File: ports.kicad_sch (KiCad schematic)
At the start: 6 parts, among them J1 PCA9865 2, J12 I2C, J2 I2S, J4 IMU, J6 Expansion

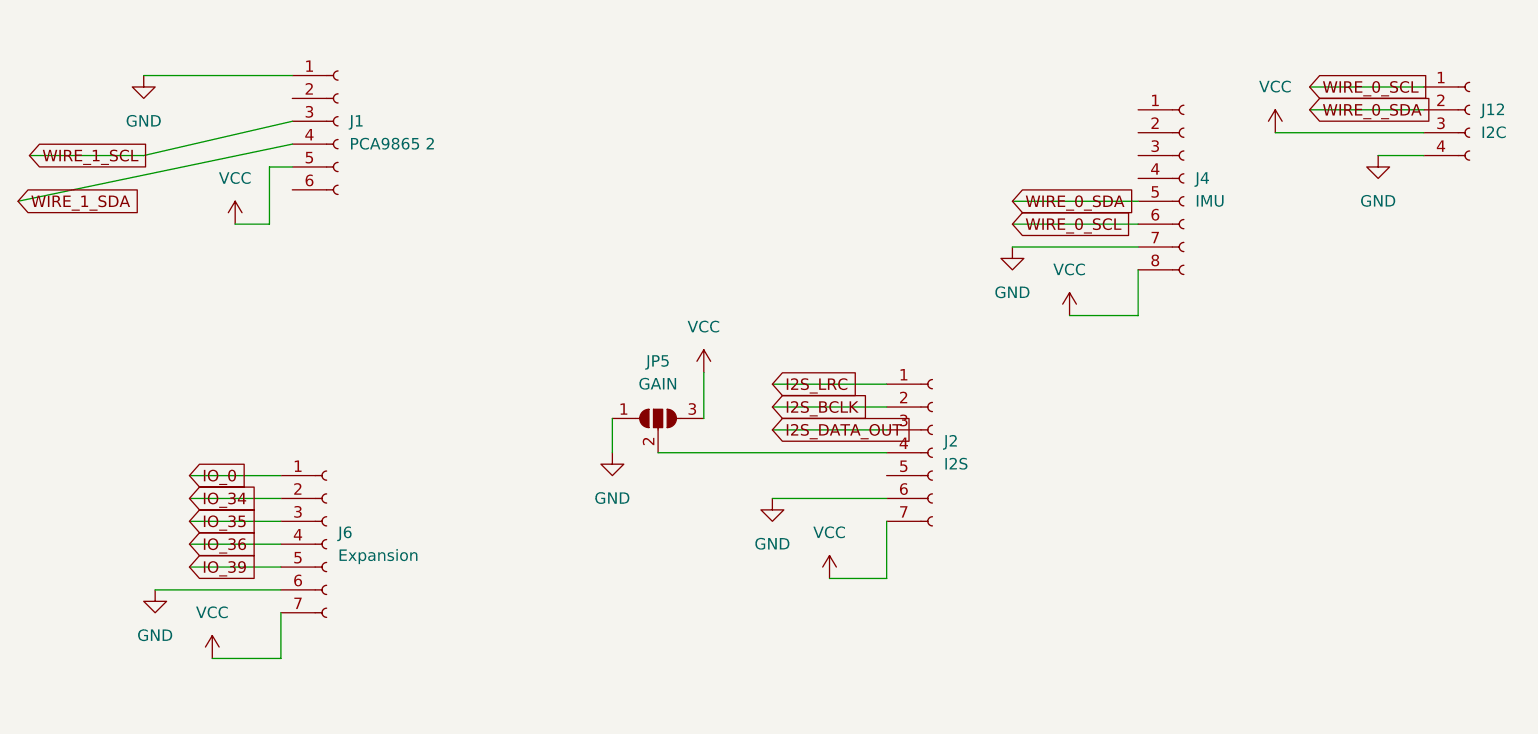
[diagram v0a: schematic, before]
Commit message: Cleaned revision 2.
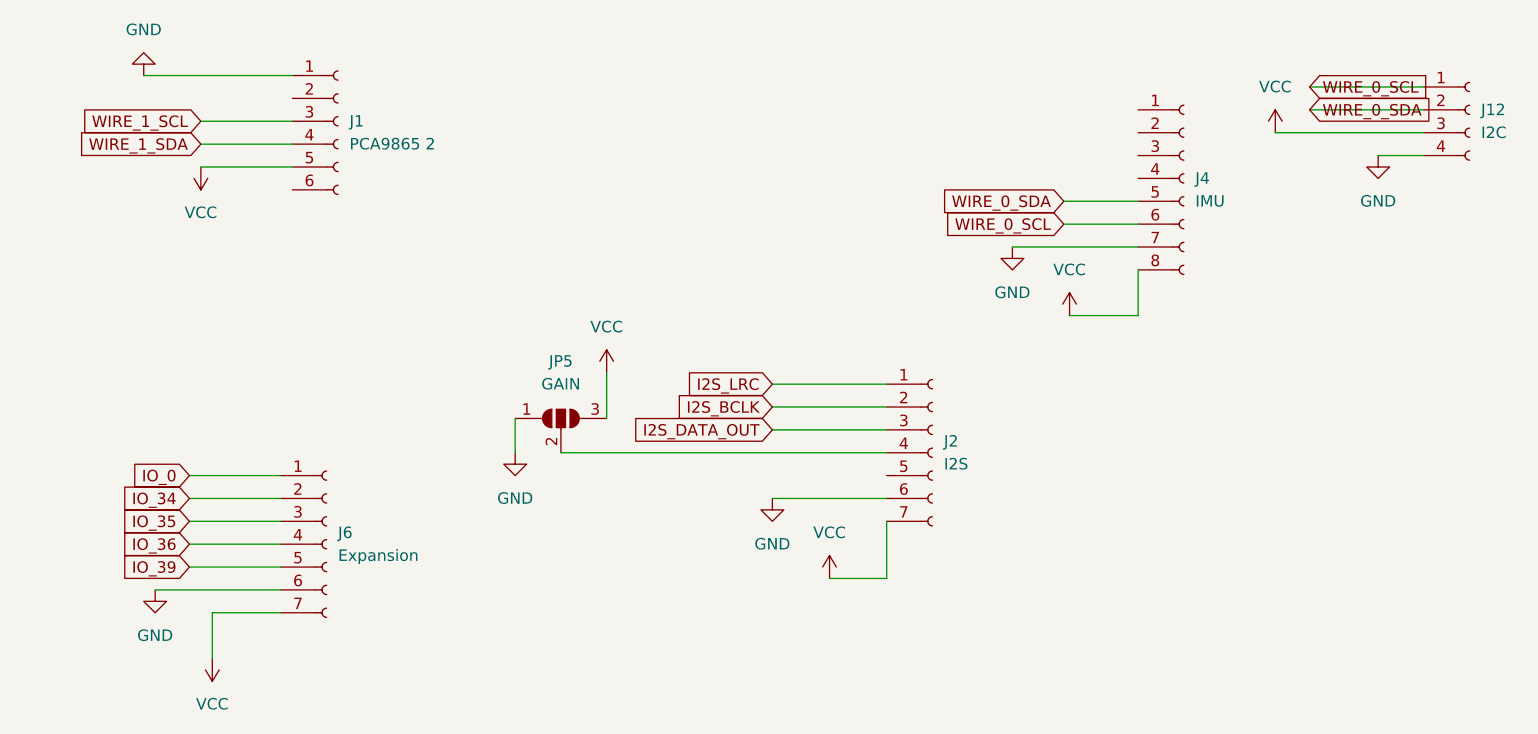
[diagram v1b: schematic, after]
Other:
- moved on the sheet: JP5
